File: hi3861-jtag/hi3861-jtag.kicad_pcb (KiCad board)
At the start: 2 copper layers, 33 x 33 mm, 9 parts, among them J1 Conn_01x12, J2 Conn_01x12, J3 Conn_ARM_JTAG_SWD_20

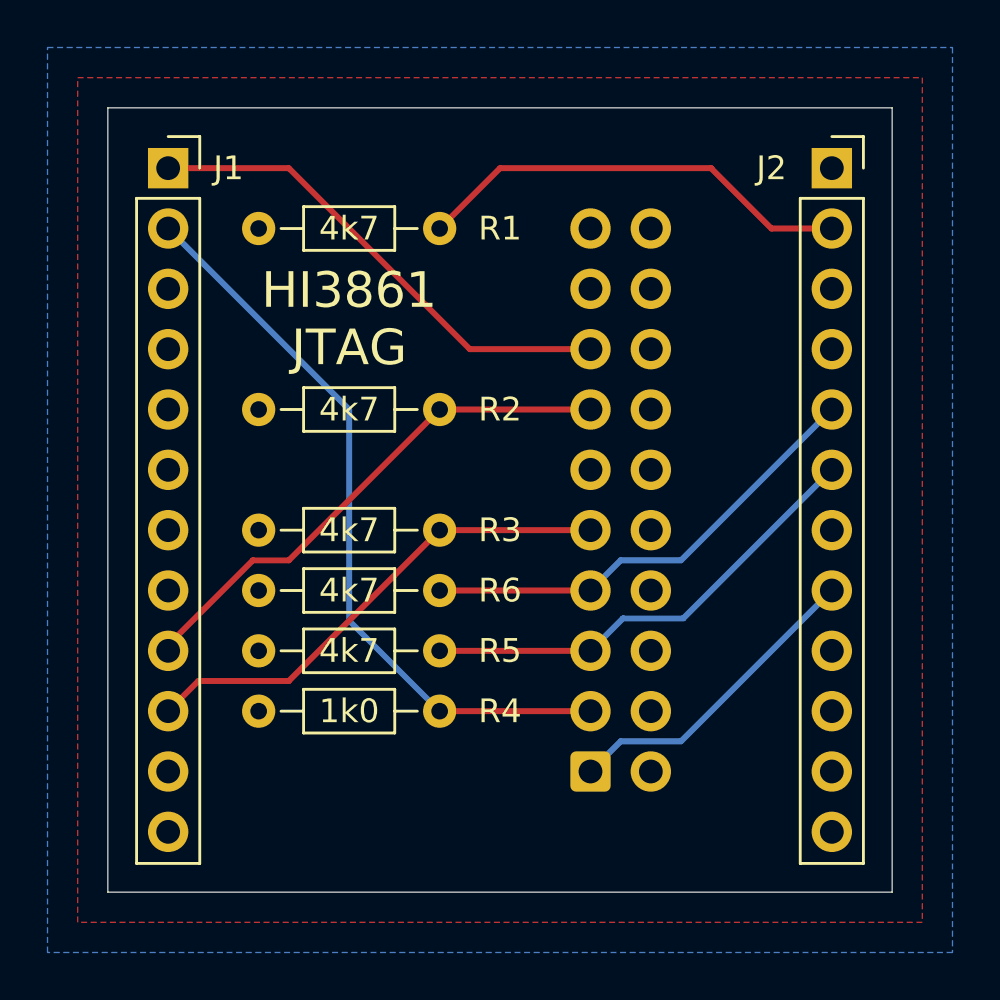
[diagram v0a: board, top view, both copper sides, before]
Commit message: updt
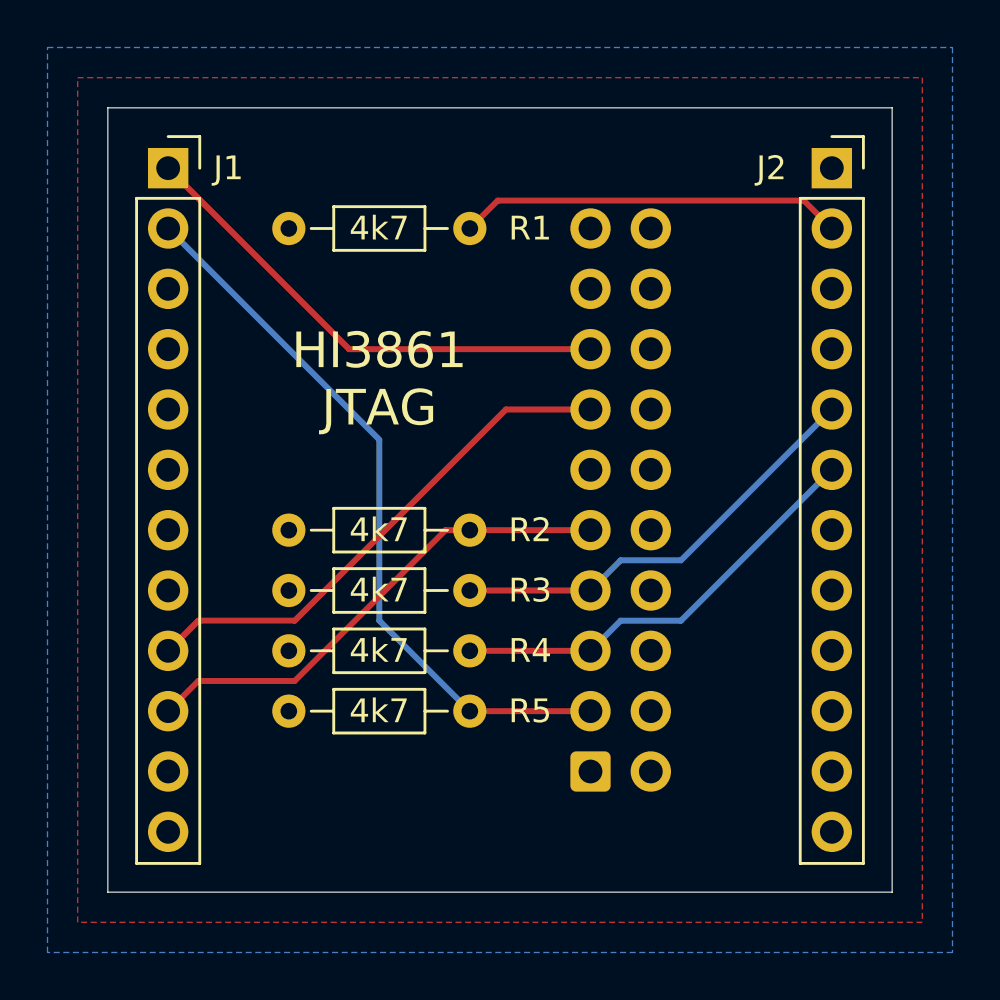
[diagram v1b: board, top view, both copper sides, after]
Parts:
- removed the R2 at (99.1, 64.8)
- removed the R5 at (99.1, 74.9)
- added R4: 4k7, Resistor_THT:R_Axial_DIN0204_L3.6mm_D1.6mm_P7.62mm_Horizontal, F.Cu at (100.3, 74.9)
- R5: renamed from R4; value 1k0 -> 4k7
- moved R1 1.27 mm to (100.3, 57.1)
- moved R2 1.27 mm to (100.3, 69.8)
- moved R3 1.27 mm to (100.3, 72.4)
- moved R5 1.27 mm to (100.3, 77.5)
- renumbered R3 to R2, R6 to R3
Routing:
- net +3V3: track 13.3 -> 0.00 mm
- net JTAG_EN: track 18.6 -> 16.2 mm
- net TMS: track 19.7 -> 18.4 mm
- net TDI: track 19.7 -> 18.4 mm
- net TRST: track 31.4 -> 30.7 mm
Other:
- board text added: "5V"
- board text added: "GND"
- board text added: "IO0"
- board text added: "IO1"
- board text added: "IO10"
- board text added: "IO11"
- board text added: "IO12"
- board text added: "IO13"
- board text added: "IO14"
- board text added: "IO2"
- board text added: "IO3"
- board text added: "IO4"
- board text added: "IO5"
- board text added: "IO7"
- board text added: "IO8"
- board text added: "IO9"
- board text added: "VIN"
